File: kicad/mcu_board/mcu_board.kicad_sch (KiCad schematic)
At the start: 31 parts, among them J1 Buttons, J10 Lights, J2 Humidity, J3 IR, J4 Power Monitor, J5 Photoresistor, J6 24V In, J7 5V Out, J8 Programmer, J9 Power Board, SW1 Reset, U1 ATmega328-P, Y1 16MHz

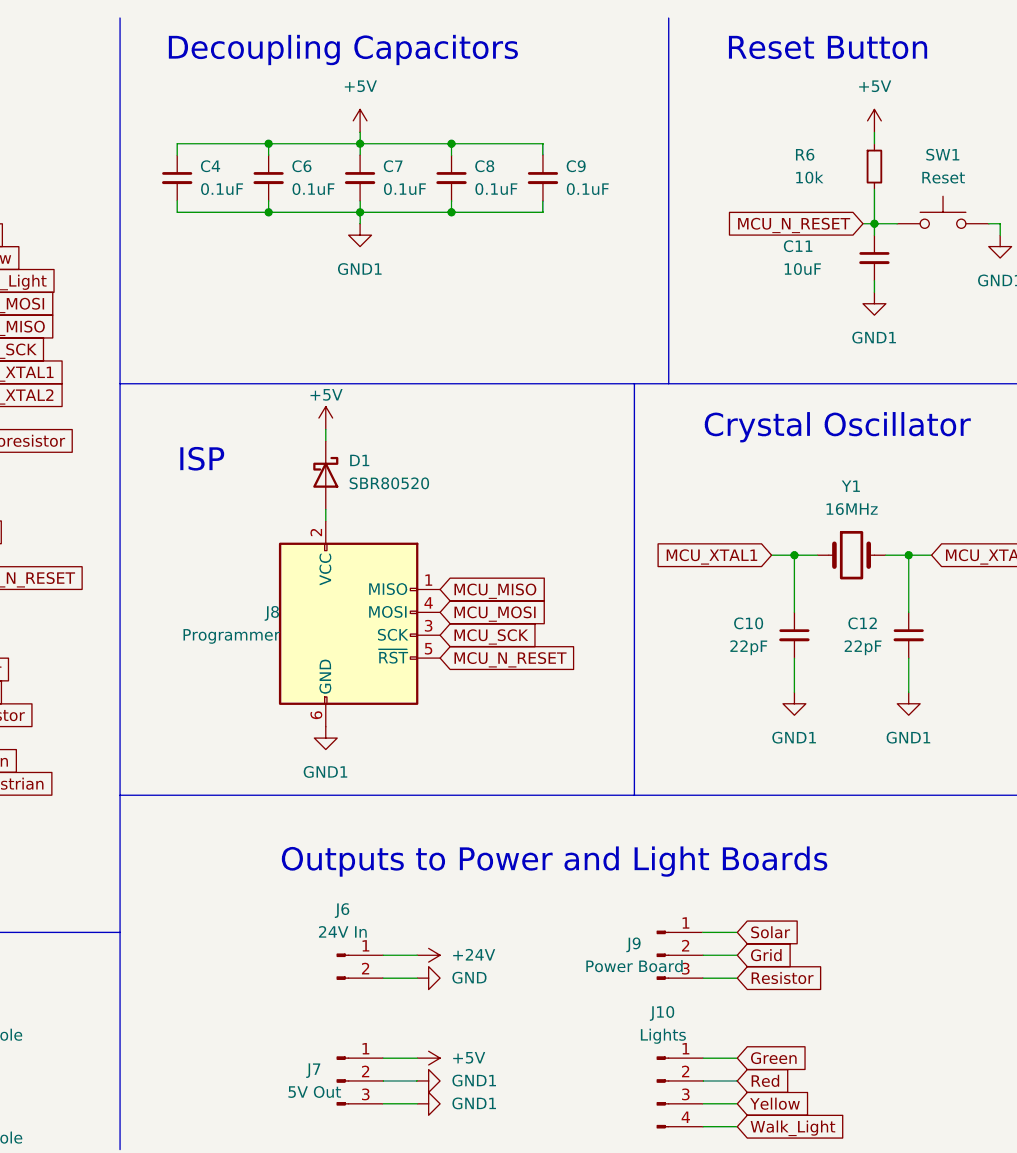
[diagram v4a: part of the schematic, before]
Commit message: finishing up MCU and adding gerbers
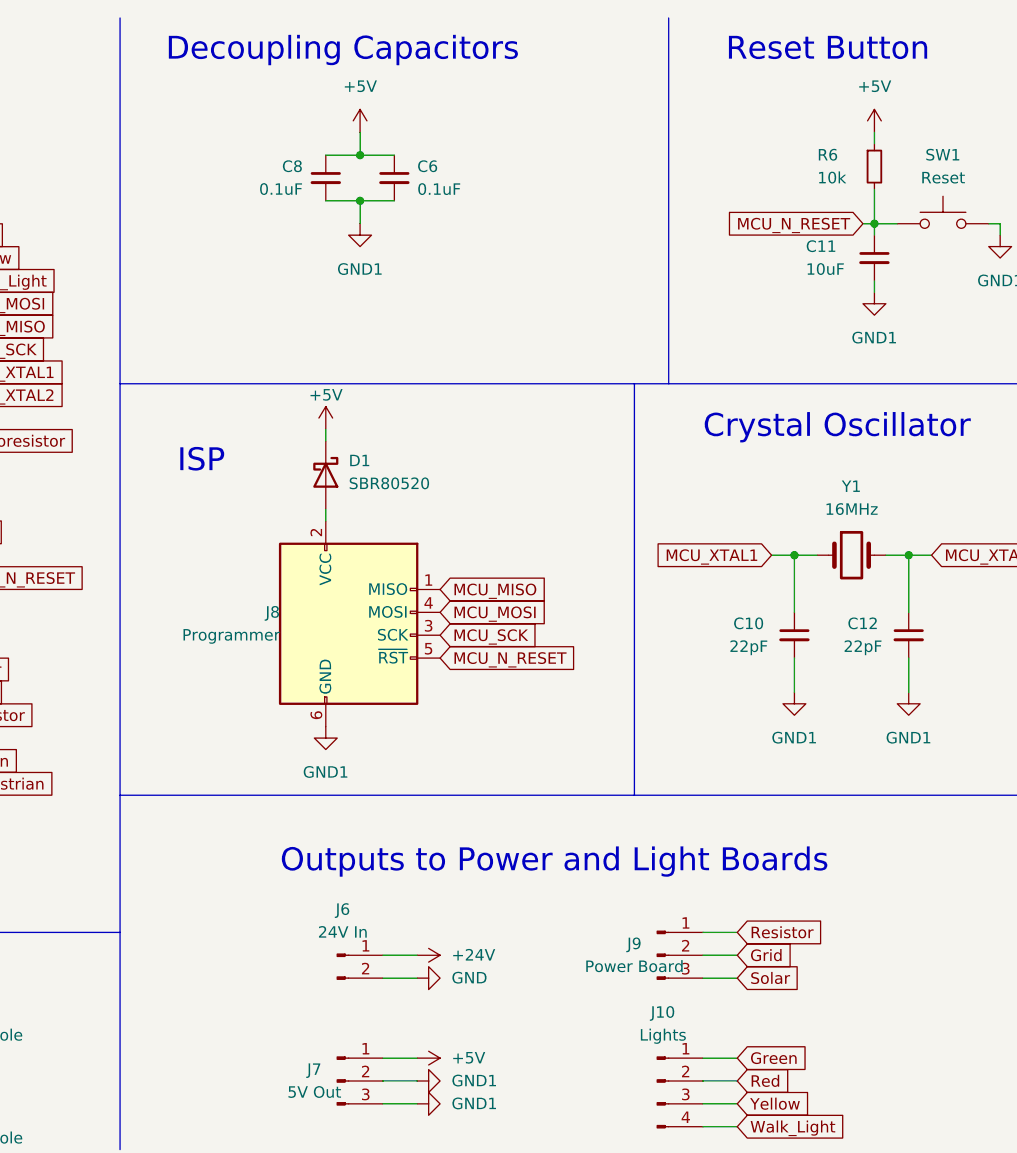
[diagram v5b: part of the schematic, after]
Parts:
- removed C4, C7, C9: 0.1uF, Capacitor_SMD:C_0603_1608Metric_Pad1.08x0.95mm_HandSolder, symbol Device:C_Small
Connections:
- net Resistor: now also J9.1 (Pin_1); no longer J9.3 (Pin_3)
- net Solar: now also J9.3 (Pin_3); no longer J9.1 (Pin_1)
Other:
- moved on the sheet: C6, C8
